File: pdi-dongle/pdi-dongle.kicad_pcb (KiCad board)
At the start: 2 copper layers, 12.7 x 10.2 mm, 6 parts, among them P101 CONN_6, P102 CONN_10

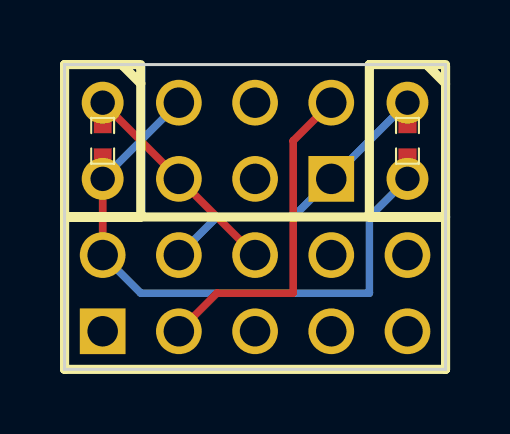
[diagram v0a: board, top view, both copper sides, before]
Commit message: new version of the PDI adapter board
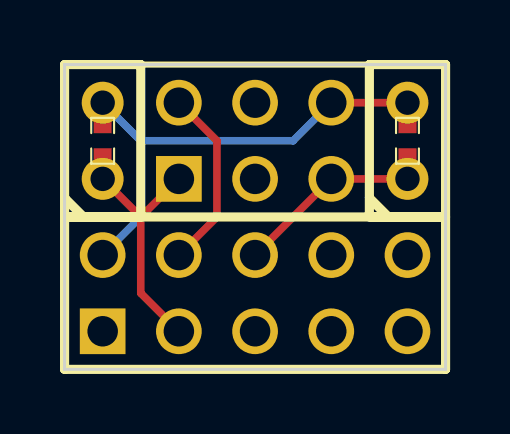
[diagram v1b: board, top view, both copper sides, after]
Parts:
- P101: moved to F.Cu
- moved C101 10.2 mm to (218.4, 153.7), turned to 90 degrees
- moved C102 10.2 mm to (208.3, 153.7), turned to 90 degrees
- moved C104 10.2 mm to (218.4, 153.7), turned to 90 degrees
- moved C105 10.2 mm to (208.3, 153.7), turned to 90 degrees
- turned P101 to 0 degrees
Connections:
- P102 pad 3: /VREF -> /PDI_D
- P102 pad 4: /PDI_D -> /VREF
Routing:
- net /VREF: track 11.2 -> 6.13 mm
- net GND: track 21.5 -> 17.2 mm
- net /PDI_D: track 10.5 -> 8.75 mm
- net /PDI_C: track 8.00 -> 6.95 mm
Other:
- board text added: "v2"
